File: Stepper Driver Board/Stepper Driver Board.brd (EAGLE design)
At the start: 40 x 29.5 mm, 30 parts, among them IC1 DRV8825PWP

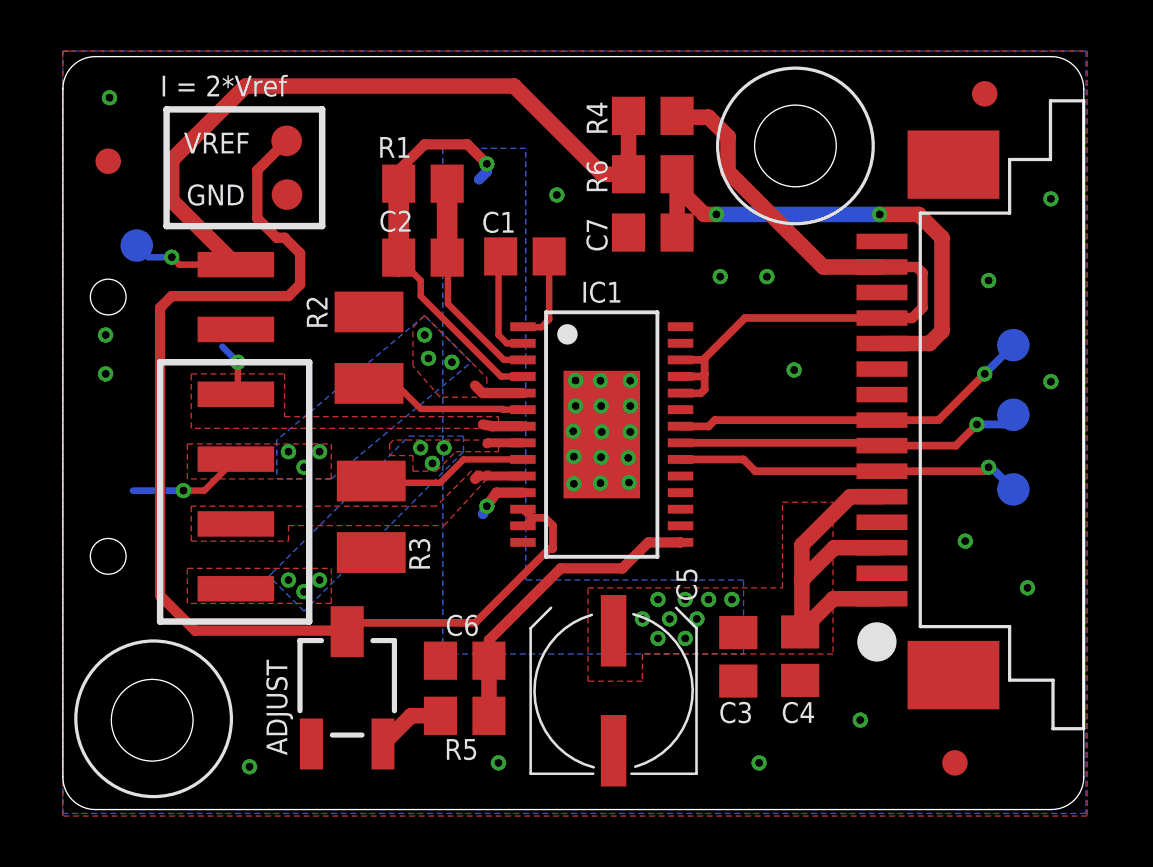
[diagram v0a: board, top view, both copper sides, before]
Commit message: BCN3D Electronics REV.E tested and manufactured
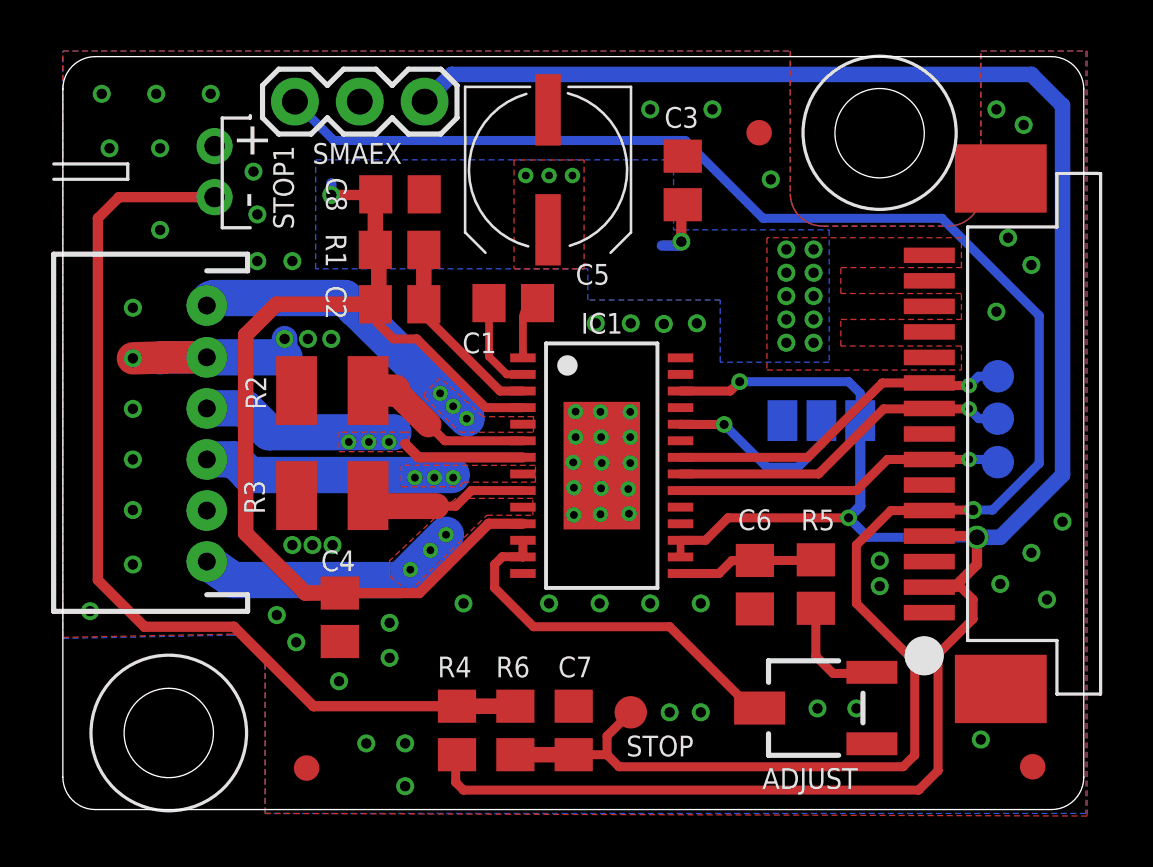
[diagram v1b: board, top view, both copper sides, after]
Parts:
- removed FFC1: FFC_15V_90G_1MM, MarcEagleParts:TE_FFC_CON1MM
- removed GND, VREF: PTR1TP12R, testpad:TP12R
- removed JP2: (no value), SparkFun-Connectors:1X06-SMD
- removed LOGO1: OSHW-LOGOL, SparkFun-Aesthetics:OSHW-LOGO-L
- removed TP1, TP2, TP3, TP8: TPB1,27, testpad:B1,27
- removed U$1: (no value), MarcEagleParts:BCN3D_LOGO
- removed U$6: (no value), MarcEagleParts:CC_LOGO
- added !EN, DIR, STEP, STOP: TPB1,27, testpad:B1,27
- added C8: 0.1uF, rcl:C0805
- added FFC2: FFC_15V_90G_1MM, MarcEagleParts:TE_FFC_CON1MM
- added MOTOR: (no value), MarcEagleParts:JST-6-PTH
- added SMAEX: (no value), SparkFun-Connectors:1X03
- added STOP1: (no value), adafruit:JST-PH-2-THM-RA
- added USTEP: (no value), jumper:SJ_2
- C3: value 0.1uF -> 100n
- moved R4 25.3 mm to (15.4, 3.10), turned to 270 degrees
- moved U$3 25.0 mm to (9.55, 1.63)
- moved R6 22.4 mm to (17.7, 3.10), turned to 270 degrees
- moved C5 20.6 mm to (19.0, 25.1), turned to 270 degrees
- moved C7 19.8 mm to (20.0, 3.10), turned to 90 degrees
- moved C3 18.8 mm to (24.3, 24.6), turned to 90 degrees
- moved ADJUST 18.4 mm to (29.5, 3.98), turned to 180 degrees
- moved C4 18.1 mm to (10.9, 7.53)
- moved R5 14.7 mm to (29.5, 8.83), turned to 90 degrees
- moved U$5 12.7 mm to (39.8, 0.76)
- moved C6 11.8 mm to (27.1, 8.81), turned to 270 degrees
- moved U$4 8.97 mm to (27.3, 26.5)
- moved U$2 3.05 mm to (38.0, 1.68)
- moved R1 2.75 mm to (13.2, 21.9)
- moved R2 2.21 mm to (10.6, 16.4), turned to 180 degrees
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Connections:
- removed net N$30: JP2.2
- new net N$4: IC1.24, USTEP.2
- net !EN: now also !EN.TP, FFC2.9; no longer FFC1.7, TP3.TP
- net +24V: now also C8.1, FFC2.11, FFC2.13, FFC2.15; no longer FFC1.1, FFC1.3, FFC1.5
- net +5V: now also FFC2.2, FFC2.4, IC1.16, IC1.17, SMAEX.1, USTEP.3; no longer FFC1.12, FFC1.14, IC1.24, IC1.25
- net A1: now also MOTOR.6; no longer JP2.4
- net A2: now also MOTOR.4; no longer JP2.3
- net B1: now also MOTOR.1; no longer JP2.5
- net B2: now also MOTOR.3; no longer JP2.6
- net DIR: now also DIR.TP, FFC2.7; no longer FFC1.6, TP1.TP
- net GND: now also C8.2, FFC2.1, FFC2.12, FFC2.14, FFC2.3, FFC2.6, FFC2.8, FFC2.GND@1, FFC2.GND@2, IC1.25, MOTOR.2, MOTOR.5, SMAEX.2, STOP1.1, USTEP.1; no longer FFC1.10, FFC1.13, FFC1.15, FFC1.2, FFC1.4, FFC1.9, FFC1.GND@1, FFC1.GND@2, GND.TP
- net N$25: now also STOP1.2; no longer JP2.1, TP8.TP
- net STEP: now also FFC2.10, STEP.TP; no longer FFC1.8, TP2.TP
- net STOP: now also FFC2.5, SMAEX.3, STOP.TP; no longer FFC1.11
- net VREF: no longer VREF.TP
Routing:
- net +5V: track 27.9 -> 107.0 mm, vias 0 -> 3
- net STOP: track 19.7 -> 74.2 mm, vias 2 -> 1
- net VREF: track 44.3 -> 15.1 mm
- net +24V: track 32.7 -> 44.0 mm, vias 11 -> 15
- net A2: track 3.77 -> 13.0 mm, vias 1 -> 3
- net B2: track 1.43 -> 9.98 mm, vias 6 -> 3
- net GND: track 0.00 -> 8.51 mm, vias 31 -> 74
- net B1: track 1.92 -> 10.3 mm, vias 0 -> 3
- net N$4: track 0.00 -> 7.51 mm, vias 0 -> 1
- net +3V3: track 12.1 -> 5.52 mm
- net A1: track 6.54 -> 12.5 mm, vias 7 -> 3
- net N$25: track 32.1 -> 37.5 mm, vias 1 -> 0
- net N$2: track 2.71 -> 4.37 mm
- net N$11: track 3.63 -> 2.56 mm
- net N$14: track 8.57 -> 7.67 mm
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- removed copper zone on layer 16, net A1
- removed copper zone on layer 16, net B2
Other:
- board text added: "+5v"
- board text added: "1/16"
- board text added: "1/32"
- board text added: "A1"
- board text added: "A2"
- board text added: "B1"
- board text added: "B2"
- board text added: "BCN3D Electronics Stepper Driver Board v1.0 Designed in Barcelona"
- board text added: "May 2015 REV_D"
- board text added: "gnd"
- board text added: "stop"
- board text removed: "BCN3D Electronics Stepper Driver Board v1.0 Designed in Barcelona ___________________ Stepper Driver - Jan 2015 Marc Cobler - REV_B ___________________"
- board text removed: "I = 2*Vref"
